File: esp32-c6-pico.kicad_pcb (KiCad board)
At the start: 4 copper layers, 20 x 29 mm, 65 parts, among them J1 USB4105-GF-A, J2 J2 GPIO / 2.00mm, J3 J3 GPIO / 2.00mm, SW1 RESET, SW2 BOOT, U1 ESP32-C6, U2 AP2112K-3.3, U3 W25Q32JVZPIQ, U4 SN74LV1T125, Y1 40MHz / CL=8pF

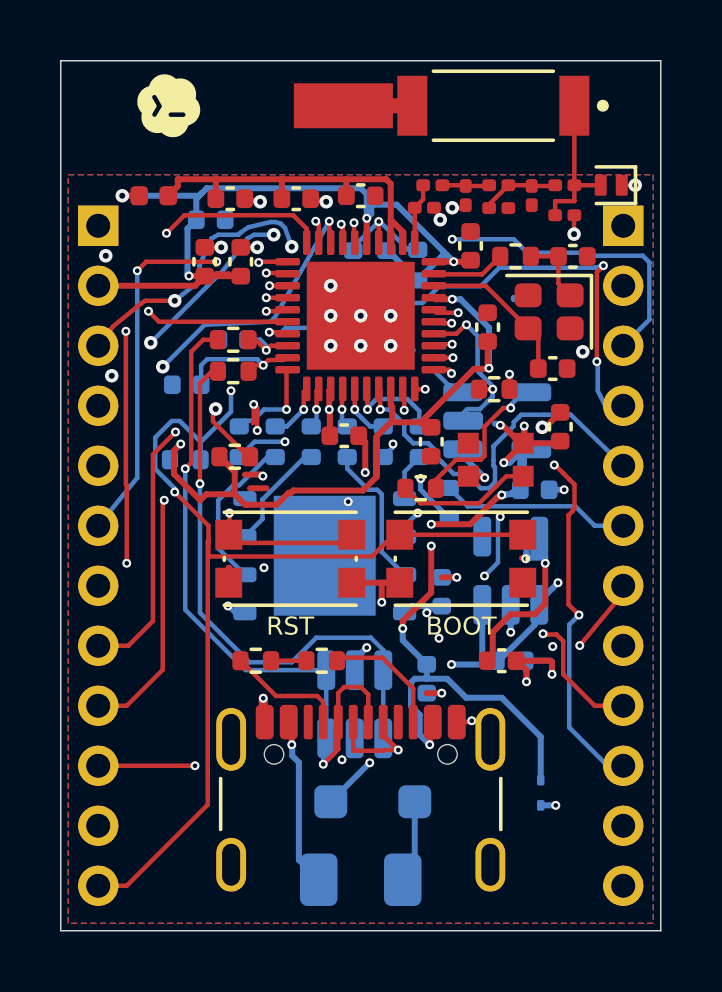
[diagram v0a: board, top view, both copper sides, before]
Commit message: optimize USB vbus routing and other
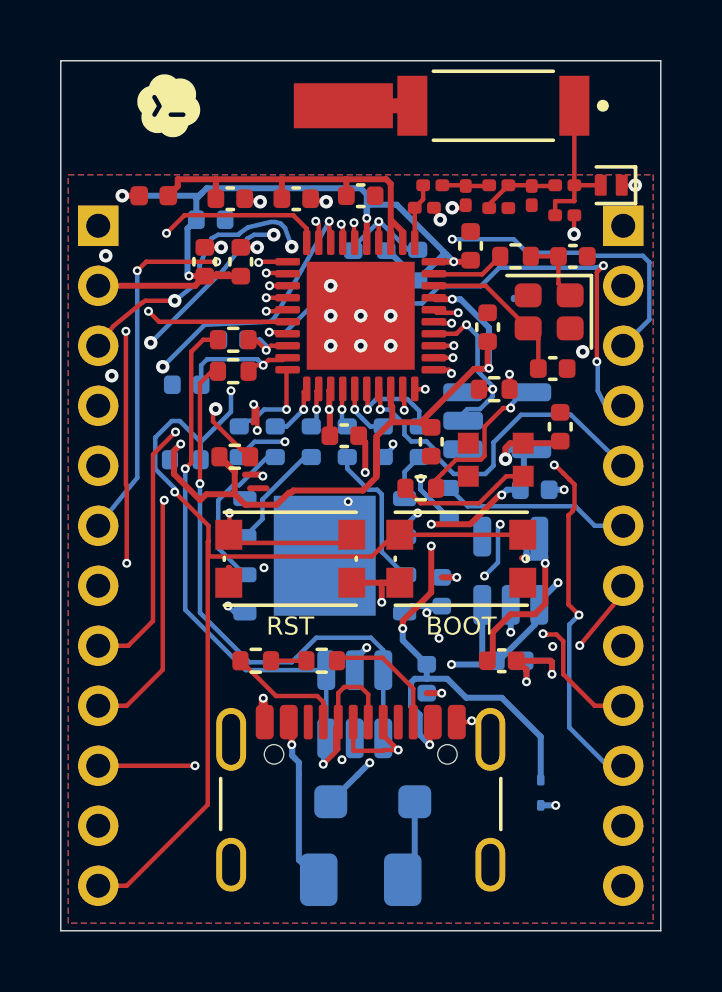
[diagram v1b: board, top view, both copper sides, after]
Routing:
- net GND: track 27.5 -> 22.6 mm, vias 38 -> 36
- net VBUS_USB: track 39.9 -> 37.2 mm, vias 10 -> 8
- net GPIO20: track 19.6 -> 18.6 mm
- net GPIO15: track 12.7 -> 12.0 mm
- net U0TXD_MCU: track 7.38 -> 6.66 mm
